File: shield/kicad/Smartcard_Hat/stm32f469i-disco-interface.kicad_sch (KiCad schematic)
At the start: 5 parts

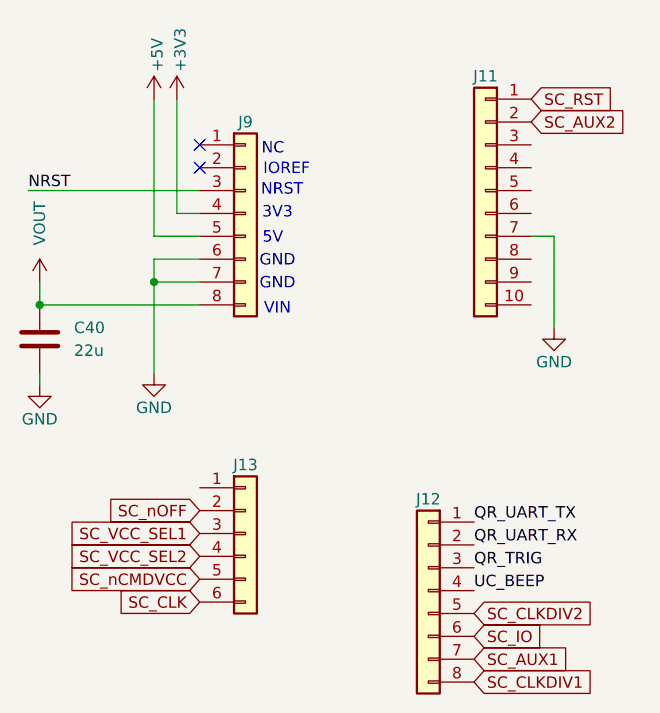
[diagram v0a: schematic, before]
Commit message: wip
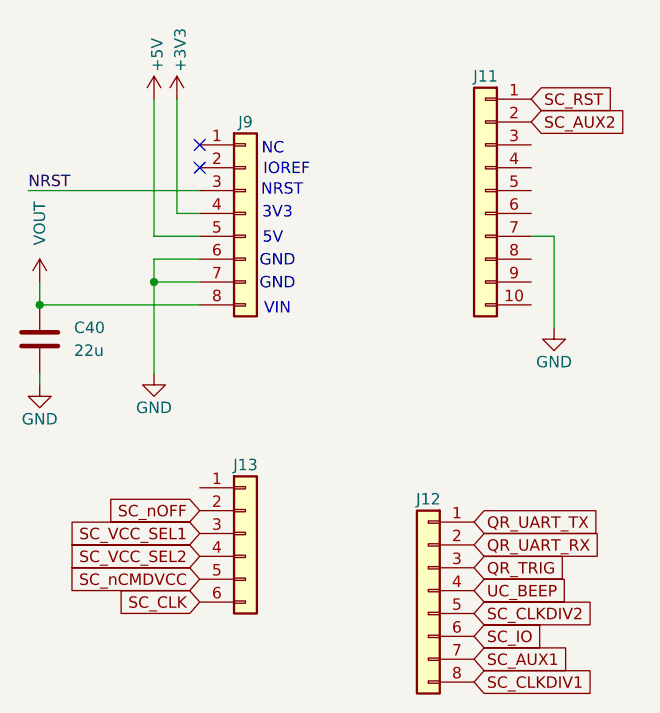
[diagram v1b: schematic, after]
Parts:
- J11: footprint Connector_PinHeader_2.54mm:PinHeader_1x10_P2.54mm_Vertical_SMD_Pin1Left -> Connector_PinHeader_2.54mm:PinHeader_1x10_P2.54mm_Vertical_SMD_Pin1Right
- J12, J9: footprint Connector_PinHeader_2.54mm:PinHeader_1x08_P2.54mm_Vertical_SMD_Pin1Left -> Connector_PinHeader_2.54mm:PinHeader_1x08_P2.54mm_Vertical_SMD_Pin1Right
- J13: footprint Connector_PinHeader_2.54mm:PinHeader_1x06_P2.54mm_Vertical_SMD_Pin1Left -> Connector_PinHeader_2.54mm:PinHeader_1x06_P2.54mm_Vertical_SMD_Pin1Right
